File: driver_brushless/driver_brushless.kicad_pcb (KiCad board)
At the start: 2 copper layers, 50 x 50 mm, 38 parts, among them U5 L6235D

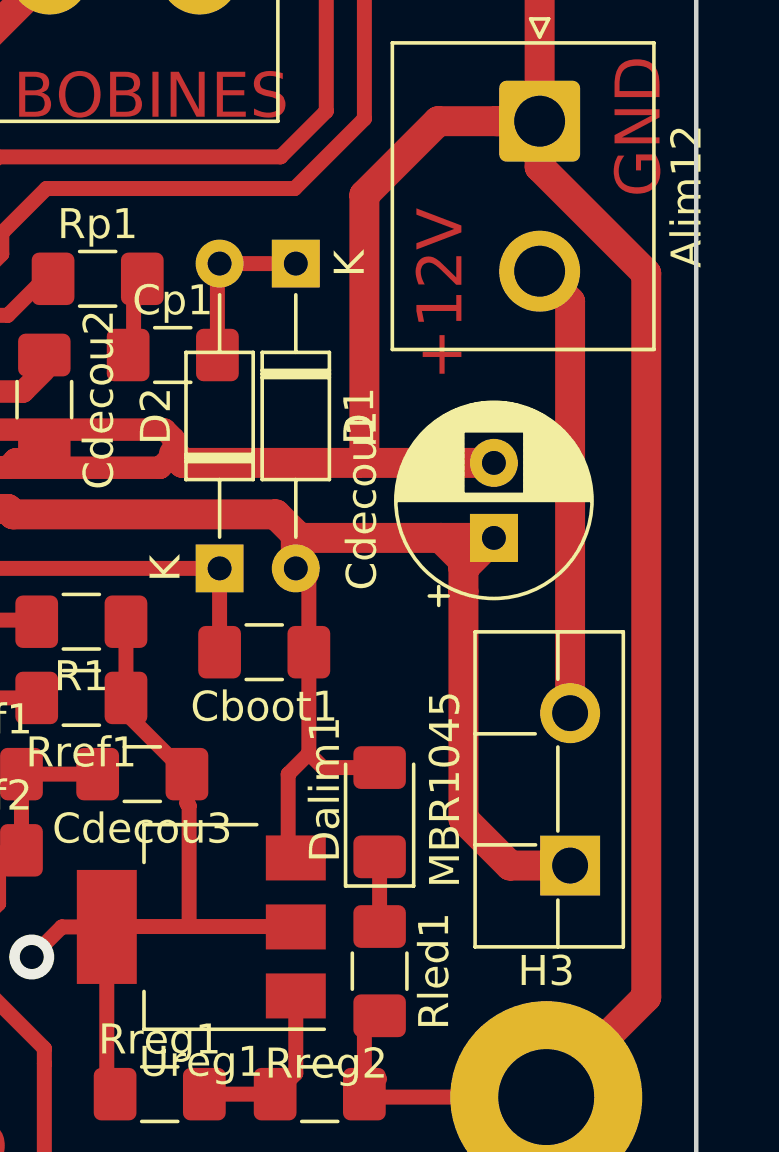
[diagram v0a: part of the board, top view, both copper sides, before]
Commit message: driver brushless
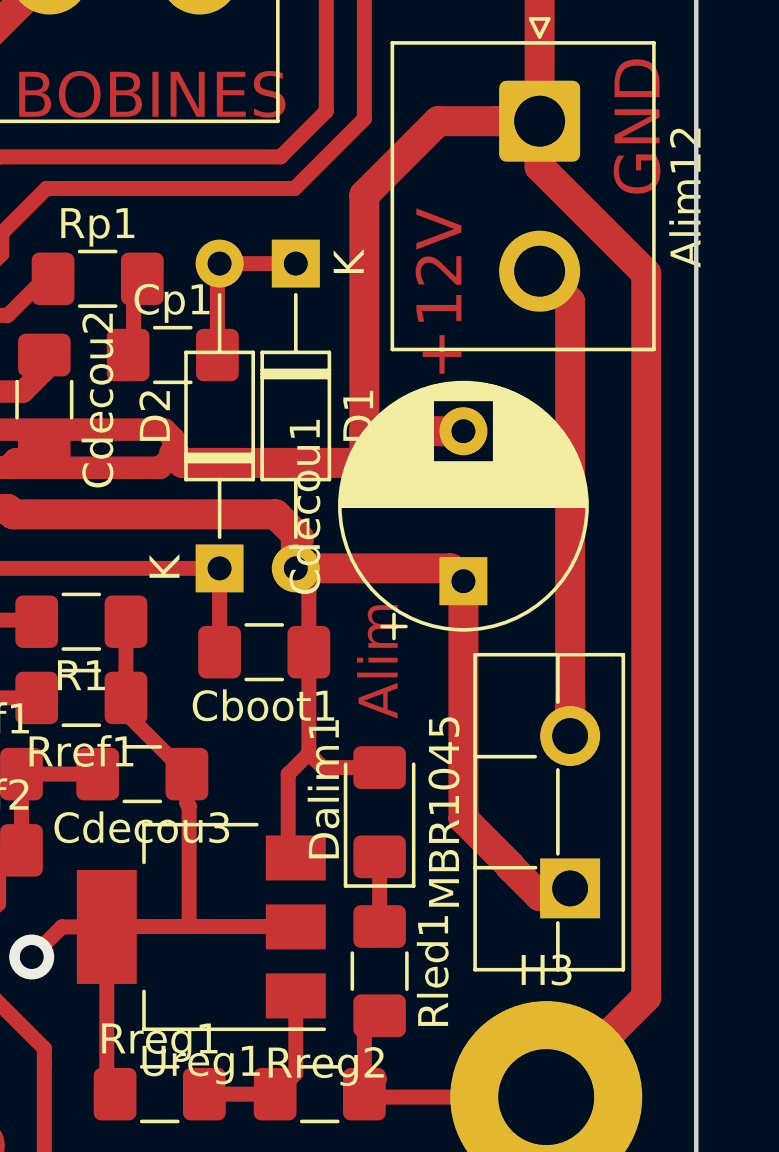
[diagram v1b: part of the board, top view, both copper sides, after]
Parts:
- Cdecou1: footprint Capacitor_THT:CP_Radial_D6.3mm_P2.50mm -> Capacitor_THT:CP_Radial_D8.0mm_P5.00mm
- Rled2: value 330 -> 680
- moved Cdecou1 1.77 mm to (142.2, 87.8)
- moved MBR1045 0.76 mm to (145.8, 98.0)
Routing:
- net +12V: track 63.2 -> 58.5 mm
- net Net-(Alim12-Pad2): track 15.2 -> 17.4 mm
- net GND: track 276.6 -> 275.3 mm
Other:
- board text added: "Alim"
